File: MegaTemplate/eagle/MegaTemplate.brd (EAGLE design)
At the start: 160 x 100 mm, 7 parts

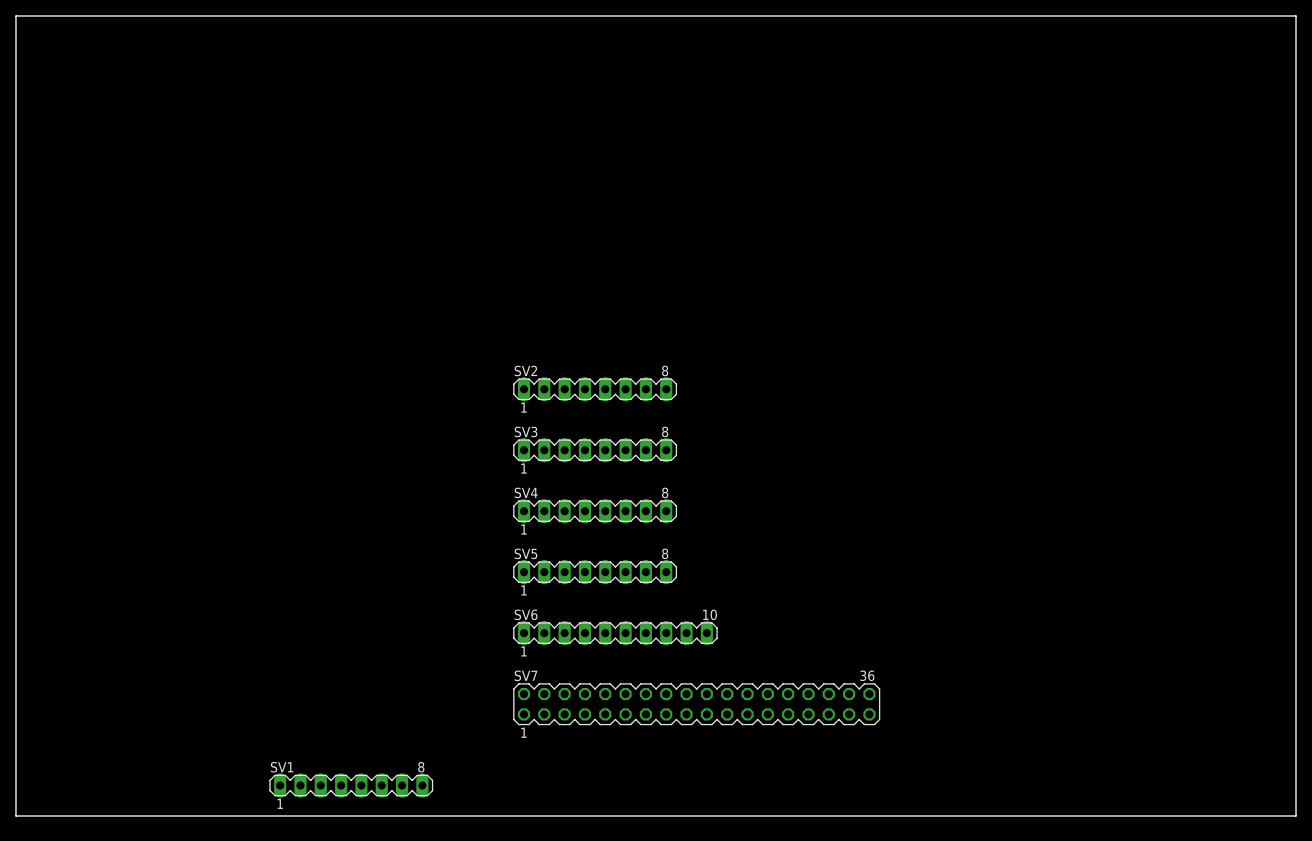
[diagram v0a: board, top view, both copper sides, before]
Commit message: Template for Arduino Mega Shields
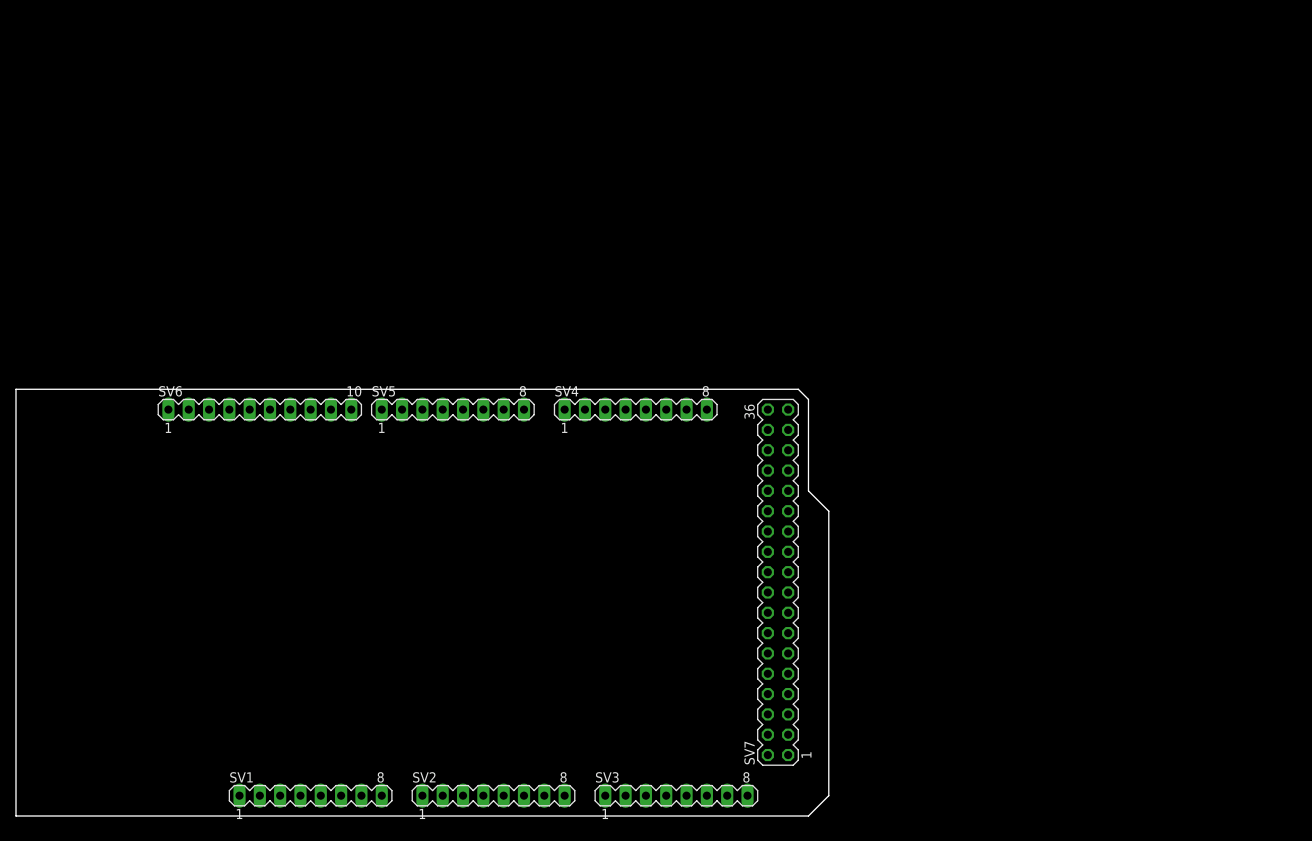
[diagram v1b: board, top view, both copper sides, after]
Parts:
- moved SV6 52.5 mm to (30.5, 50.8)
- moved SV2 52.4 mm to (59.7, 2.54)
- moved SV3 44.4 mm to (82.5, 2.54)
- moved SV5 27.0 mm to (54.6, 50.8)
- moved SV7 18.3 mm to (95.2, 29.2), turned to 90 degrees
- moved SV4 13.7 mm to (77.5, 50.8)
- moved SV1 5.24 mm to (36.8, 2.54)
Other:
- board size 160 x 100 mm -> 101.6 x 53.3 mm
